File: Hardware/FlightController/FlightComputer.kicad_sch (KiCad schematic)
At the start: 1 part, among them U2 STM32H753VITx

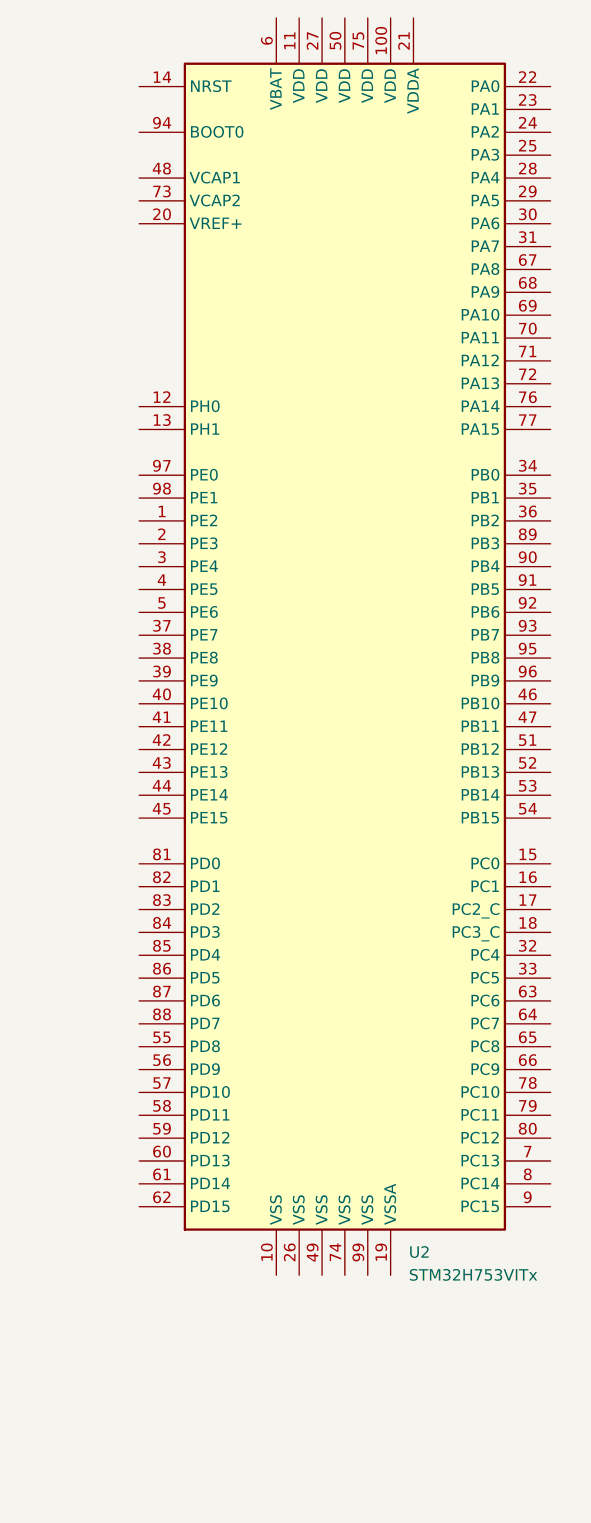
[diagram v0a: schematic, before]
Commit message: Add ICM-42670-P symbol and schematic
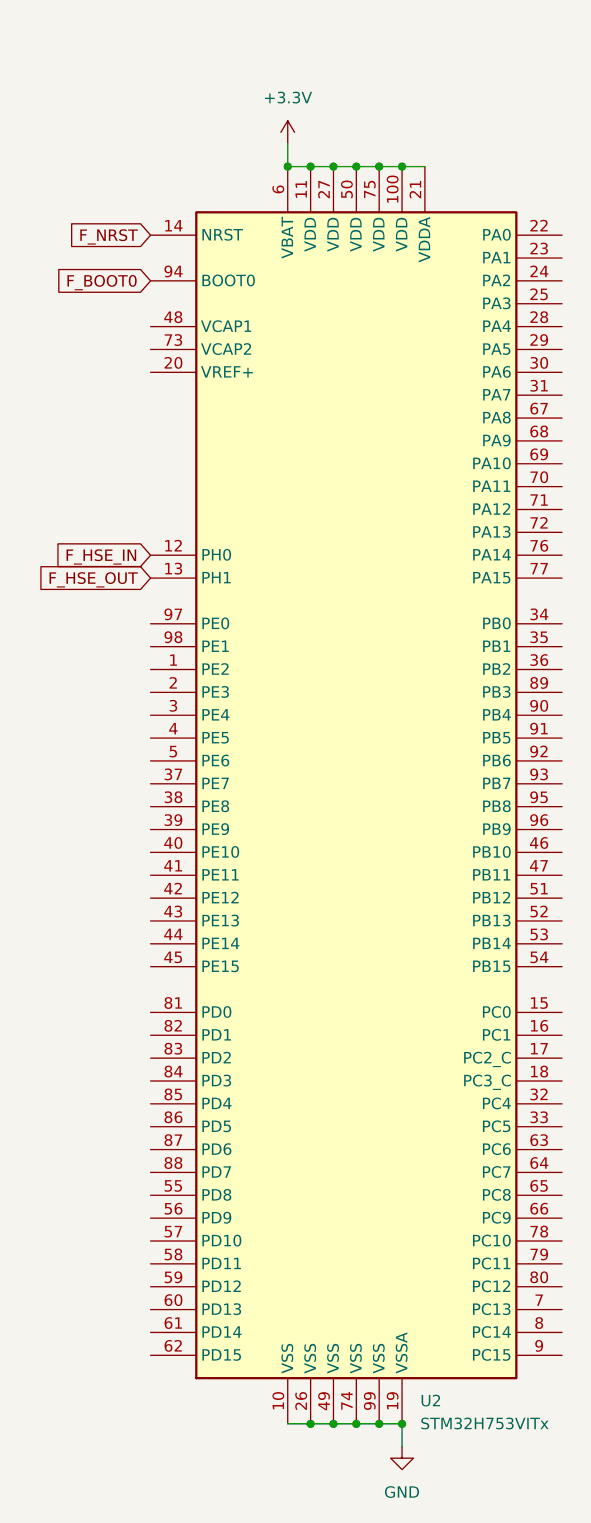
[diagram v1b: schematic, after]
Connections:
- net GND: now reaches U2.10 (VSS)
- net GND: now also U2.19 (VSSA), U2.26 (VSS), U2.49 (VSS), U2.74 (VSS), U2.99 (VSS)
- net +3V3: now reaches U2.100 (VDD)
- net +3V3: now also U2.11 (VDD), U2.21 (VDDA), U2.27 (VDD), U2.50 (VDD), U2.6 (VBAT), U2.75 (VDD)
- net F_HSE_IN: now reaches U2.12 (PH0)
- net F_HSE_OUT: now reaches U2.13 (PH1)
- net F_NRST: now reaches U2.14 (NRST)
- net F_BOOT0: now reaches U2.94 (BOOT0)
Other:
- moved on the sheet: U2
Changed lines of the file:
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@@
 (kicad_sch (version 20211123) (generator eeschema)
   (paper "A4")
-  (symbol (lib_id "MCU_ST_STM32H7:STM32H753VITx") (at 135.89 91.44 0) (unit 1)
+  (junction (at 137.16 179.07) (diameter 0) (color 0 0 0 0)
+  )
+  (junction (at 132.08 179.07) (diameter 0) (color 0 0 0 0)
+  )
+  (junction (at 139.7 39.37) (diameter 0) (color 0 0 0 0)
+  )
+  (junction (at 139.7 179.07) (diameter 0) (color 0 0 0 0)
+  )
+  (junction (at 137.16 39.37) (diameter 0) (color 0 0 0 0)
+  )
+  (junction (at 132.08 39.37) (diameter 0) (color 0 0 0 0)
+  )
+  (junction (at 134.62 179.07) (diameter 0) (color 0 0 0 0)
+  )
+  (junction (at 142.24 179.07) (diameter 0) (color 0 0 0 0)
+  )
+  (junction (at 142.24 39.37) (diameter 0) (color 0 0 0 0)
+  )
+  (junction (at 129.54 39.37) (diameter 0) (color 0 0 0 0)
+  )
+  (junction (at 134.62 39.37) (diameter 0) (color 0 0 0 0)
+  )
+  (wire (pts (xy 132.08 179.07) (xy 134.62 179.07))
+    (stroke (width 0) (type default) (color 0 0 0 0))
+  )
+  (wire (pts (xy 134.62 179.07) (xy 137.16 179.07))
+    (stroke (width 0) (type default) (color 0 0 0 0))
+  )
+  (wire (pts (xy 134.62 39.37) (xy 137.16 39.37))
+    (stroke (width 0) (type default) (color 0 0 0 0))
+  )
+  (wire (pts (xy 142.24 179.07) (xy 142.24 181.61))
+    (stroke (width 0) (type default) (color 0 0 0 0))
+  )
+  (wire (pts (xy 129.54 179.07) (xy 132.08 179.07))
+    (stroke (width 0) (type default) (color 0 0 0 0))
+  )
+  (wire (pts (xy 137.16 179.07) (xy 139.7 179.07))
+    (stroke (width 0) (type default) (color 0 0 0 0))
+  )
+  (wire (pts (xy 132.08 39.37) (xy 134.62 39.37))
+    (stroke (width 0) (type default) (color 0 0 0 0))
+  )
+  (wire (pts (xy 137.16 39.37) (xy 139.7 39.37))
+    (stroke (width 0) (type default) (color 0 0 0 0))
+  )
+  (wire (pts (xy 129.54 36.83) (xy 129.54 39.37))
+    (stroke (width 0) (type default) (color 0 0 0 0))
+  )
+  (wire (pts (xy 139.7 39.37) (xy 142.24 39.37))
+    (stroke (width 0) (type default) (color 0 0 0 0))
+  )
+  (wire (pts (xy 139.7 179.07) (xy 142.24 179.07))
+    (stroke (width 0) (type default) (color 0 0 0 0))
+  )
+  (wire (pts (xy 129.54 39.37) (xy 132.08 39.37))
+    (stroke (width 0) (type default) (color 0 0 0 0))
+  )
+  (wire (pts (xy 142.24 39.37) (xy 144.78 39.37))
+    (stroke (width 0) (type default) (color 0 0 0 0))
+  )
+  (global_label "F_BOOT0" (shape input) (at 114.3 52.07 180) (fields_autoplaced)
+    (effects (font (size 1.27 1.27)) (justify right))
+    (property "Intersheet References" "${INTERSHEET_REFS}" (id 0) (at 103.7226 51.9906 0)
+      (effects (font (size 1.27 1.27)) (justify right) hide)
+    )
+  )
+  (global_label "F_HSE_OUT" (shape input) (at 114.3 85.09 180) (fields_autoplaced)
+    (effects (font (size 1.27 1.27)) (justify right))
+    (property "Intersheet References" "${INTERSHEET_REFS}" (id 0) (at 101.5455 85.0106 0)
+      (effects (font (size 1.27 1.27)) (justify right) hide)
+    )
+  )
+  (global_label "F_HSE_IN" (shape input) (at 114.3 82.55 180) (fields_autoplaced)
+    (effects (font (size 1.27 1.27)) (justify right))
+    (property "Intersheet References" "${INTERSHEET_REFS}" (id 0) (at 103.2388 82.4706 0)
+      (effects (font (size 1.27 1.27)) (justify right) hide)
+    )
+  )
+  (global_label "F_NRST" (shape input) (at 114.3 46.99 180) (fields_autoplaced)
+    (effects (font (size 1.27 1.27)) (justify right))
+    (property "Intersheet References" "${INTERSHEET_REFS}" (id 0) (at 105.0531 46.9106 0)
+      (effects (font (size 1.27 1.27)) (justify right) hide)
+    )
+  )
+  (symbol (lib_id "power:GND") (at 142.24 181.61 0) (unit 1)
     (in_bom yes) (on_board yes) (fields_autoplaced)
-    (property "Reference" "U2" (id 0) (at 142.9894 160.02 0)
+    (property "Reference" "#PWR?" (id 0) (at 142.24 187.96 0)
+      (effects (font (size 1.27 1.27)) hide)
+    )
+    (property "Value" "GND" (id 1) (at 142.24 186.69 0))
+    (property "Footprint" "" (id 2) (at 142.24 181.61 0)
+      (effects (font (size 1.27 1.27)) hide)
+    )
+    (property "Datasheet" "" (id 3) (at 142.24 181.61 0)
+      (effects (font (size 1.27 1.27)) hide)
+    )
+    (pin "1")
+  )
+  (symbol (lib_id "MCU_ST_STM32H7:STM32H753VITx") (at 137.16 107.95 0) (unit 1)
+    (in_bom yes) (on_board yes) (fields_autoplaced)
+    (property "Reference" "U2" (id 0) (at 144.2594 176.53 0)
       (effects (font (size 1.27 1.27)) (justify left))
     )
-    (property "Value" "STM32H753VITx" (id 1) (at 142.9894 162.56 0)
+    (property "Value" "STM32H753VITx" (id 1) (at 144.2594 179.07 0)
       (effects (font (size 1.27 1.27)) (justify left))
     )
-    (property "Footprint" "Package_QFP:LQFP-100_14x14mm_P0.5mm" (id 2) (at 118.11 157.48 0)
-      (effects (font (size 1.27 1.27)) (justify right) hide)
-    )
-    (property "Datasheet" "http://www.st.com/st-web-ui/static/active/en/resource/technical/document/datasheet/DM00388325.pdf" (id 3) (at 135.89 91.44 0)
+    (property "Footprint" "Package_QFP:LQFP-100_14x14mm_P0.5mm" (id 2) (at 119.38 173.99 0)
+      (effects (font (size 1.27 1.27)) (justify right) hide)
+    )
+    (property "Datasheet" "http://www.st.com/st-web-ui/static/active/en/resource/technical/document/datasheet/DM00388325.pdf" (id 3) (at 137.16 107.95 0)
       (effects (font (size 1.27 1.27)) hide)
     )
@@
     (pin "99")
   )
+  (symbol (lib_id "power:+3.3V") (at 129.54 36.83 0) (unit 1)
+    (in_bom yes) (on_board yes) (fields_autoplaced)
+    (property "Reference" "#PWR?" (id 0) (at 129.54 40.64 0)
+      (effects (font (size 1.27 1.27)) hide)
+    )
+    (property "Value" "+3.3V" (id 1) (at 129.54 31.75 0))
+    (property "Footprint" "" (id 2) (at 129.54 36.83 0)
+      (effects (font (size 1.27 1.27)) hide)
+    )
+    (property "Datasheet" "" (id 3) (at 129.54 36.83 0)
+      (effects (font (size 1.27 1.27)) hide)
+    )
+    (pin "1")
+  )
 )
